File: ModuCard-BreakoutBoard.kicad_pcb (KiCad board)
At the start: 2 copper layers, 41 parts, among them J1 09031967921, J10 USB_C_Receptacle_USB2.0_16P, J9 RJ45_LED_Shielded, Q1 AO3401A, Q2 AO3401A, SW1 SW_SPDT_321, SW2 SW_SPDT_321, SW3 SW_SPDT_321, U1 XL4015, U2 IP4234CZ6,115

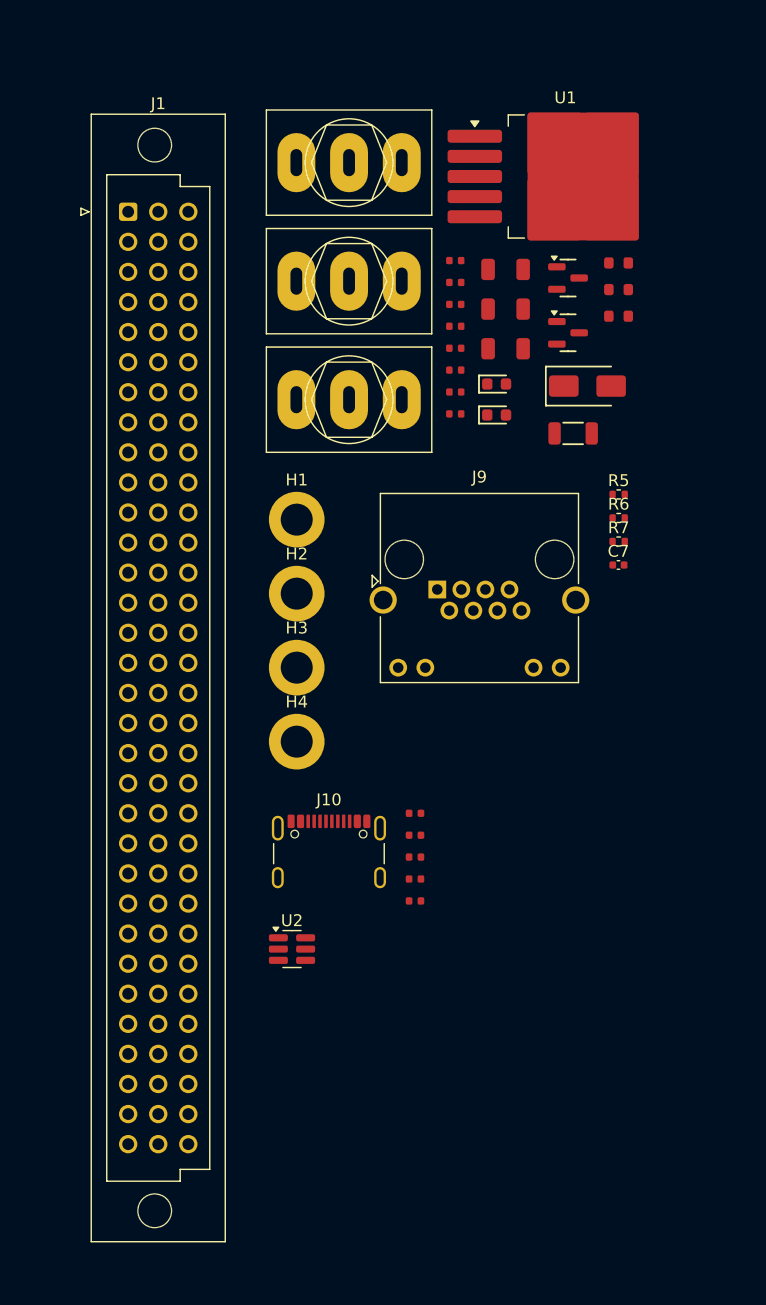
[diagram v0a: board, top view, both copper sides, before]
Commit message: Create fundamental layout
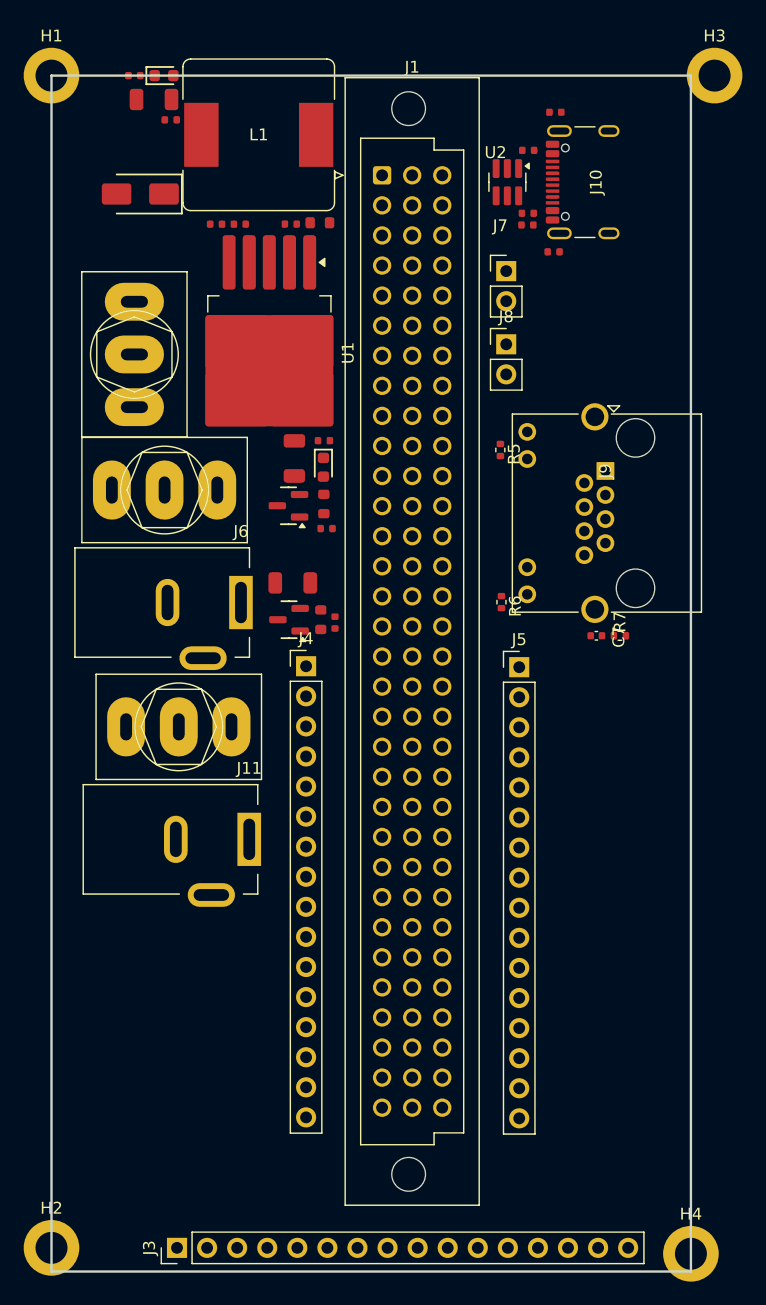
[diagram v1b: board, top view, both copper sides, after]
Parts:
- added J11: Barrel_Jack_Switch, Connector_BarrelJack:BarrelJack_Kycon_KLDX-0202-xC_Horizontal, F.Cu at (31.2, 78.5)
- added J3: Conn_01x16_Pin, Connector_PinHeader_2.54mm:PinHeader_1x16_P2.54mm_Vertical, F.Cu at (25.1, 113.0)
- added J4: Conn_01x16_Pin, Connector_PinHeader_2.54mm:PinHeader_1x16_P2.54mm_Vertical, F.Cu at (36.0, 63.9)
- added J5: Conn_01x16_Pin, Connector_PinHeader_2.54mm:PinHeader_1x16_P2.54mm_Vertical, F.Cu at (54.0, 64.0)
- added J6: Barrel_Jack_Switch, Connector_BarrelJack:BarrelJack_Kycon_KLDX-0202-xC_Horizontal, F.Cu at (30.5, 58.5)
- added J7: Conn_01x02_Pin, Connector_PinHeader_2.54mm:PinHeader_1x02_P2.54mm_Vertical, F.Cu at (52.9, 30.5)
- added J8: Conn_01x02_Pin, Connector_PinHeader_2.54mm:PinHeader_1x02_P2.54mm_Vertical, F.Cu at (52.9, 36.7)
- L1: value 4.7uH,25mA -> 40uH; footprint PCM_JLCPCB:L_1206 -> Inductor_SMD:L_Bourns_SRR1260
- moved U2 67.3 mm to (53.0, 23.0), turned to -90 degrees
- moved R9 62.3 mm to (54.8, 20.3), turned to 180 degrees
- moved J10 61.9 mm to (60.5, 23.0), turned to 90 degrees
- moved H3 61.2 mm to (70.5, 14.0)
- moved C8 60.4 mm to (57.1, 17.1), turned to 180 degrees
- moved H2 59.0 mm to (14.5, 113.0)
- moved R10 58.8 mm to (54.7, 25.6), turned to 180 degrees
- moved H4 54.6 mm to (68.5, 113.5)
- moved R8 52.4 mm to (56.9, 28.9), turned to 180 degrees
- moved C9 52.4 mm to (54.7, 26.6), turned to 180 degrees
- moved H1 42.8 mm to (14.5, 14.0)
- moved D2 41.1 mm to (22.0, 24.0), turned to 180 degrees
- moved SW2 40.3 mm to (25.2, 69.0)
- moved D5 40.1 mm to (24.0, 14.0)
- moved Q1 37.3 mm to (34.6, 60.0), turned to 180 degrees
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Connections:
- R5 pad 2: +12V_DC_JACK -> +12V
- R6 pad 2: +12V_DC_JACK -> +12V
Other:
- board outline added: 54 x 101 mm
